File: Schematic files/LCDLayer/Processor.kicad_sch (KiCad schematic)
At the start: 16 parts, among them SW1 SW_SPDT, U5 STM32F103C8Tx, Y1 16MHz

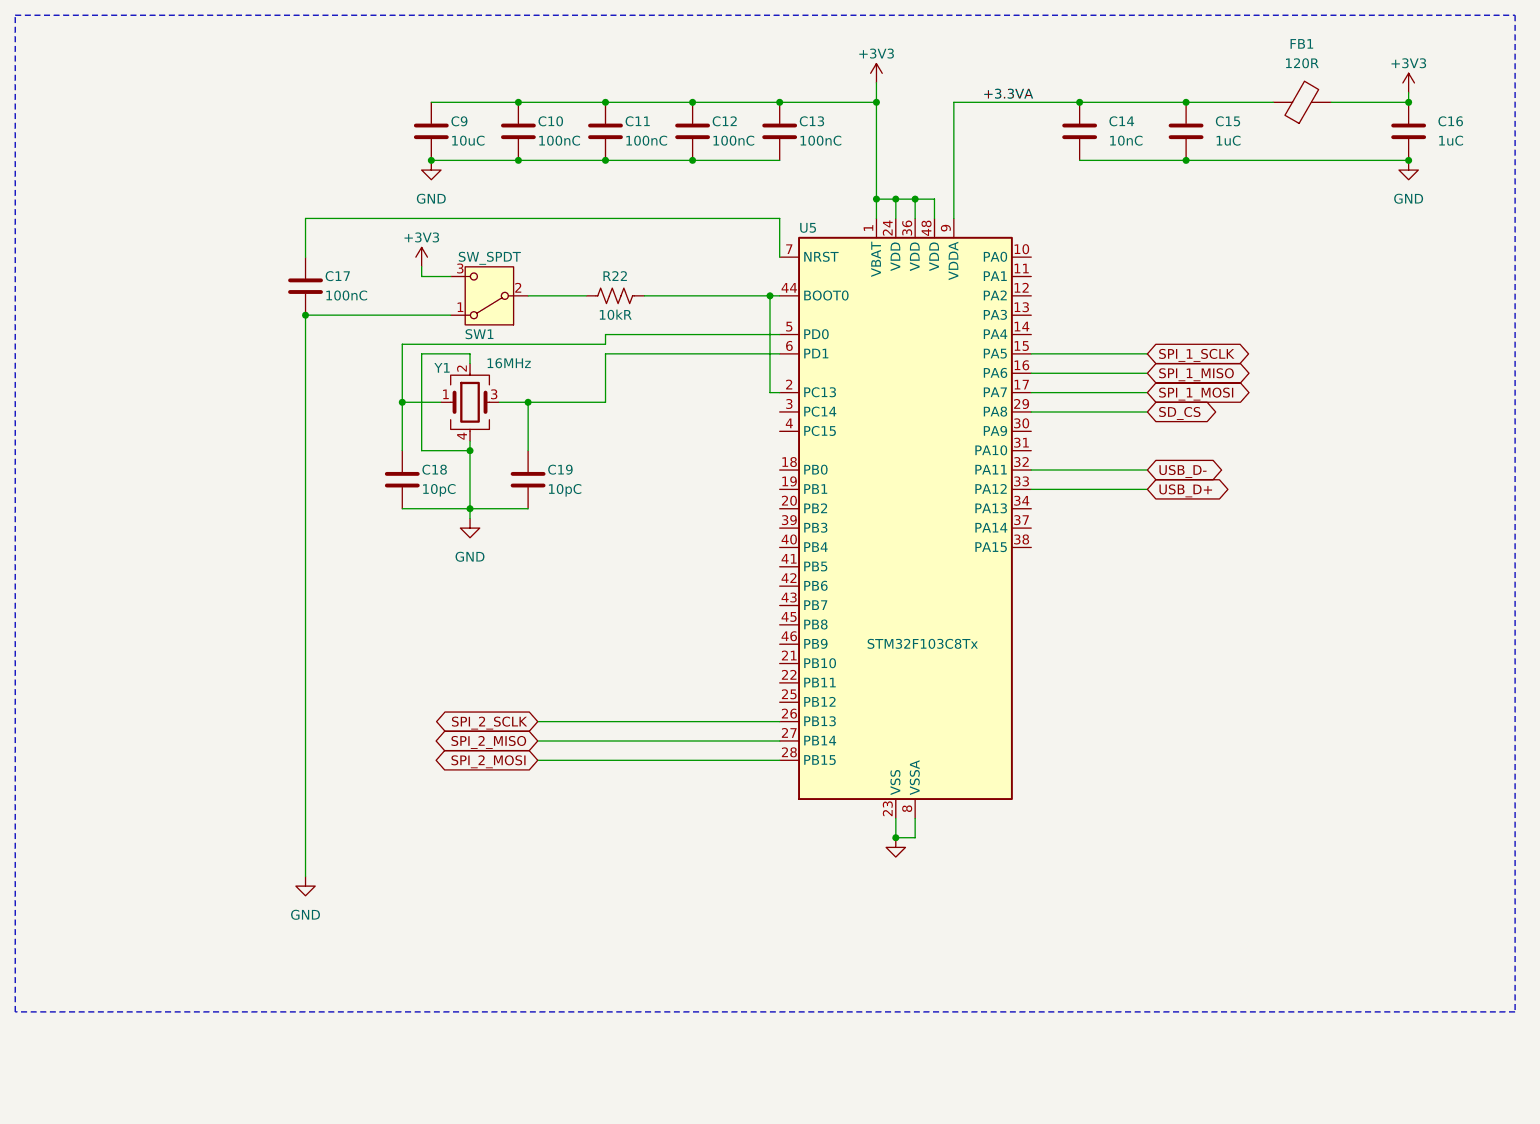
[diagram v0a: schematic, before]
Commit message: Finished Schematic
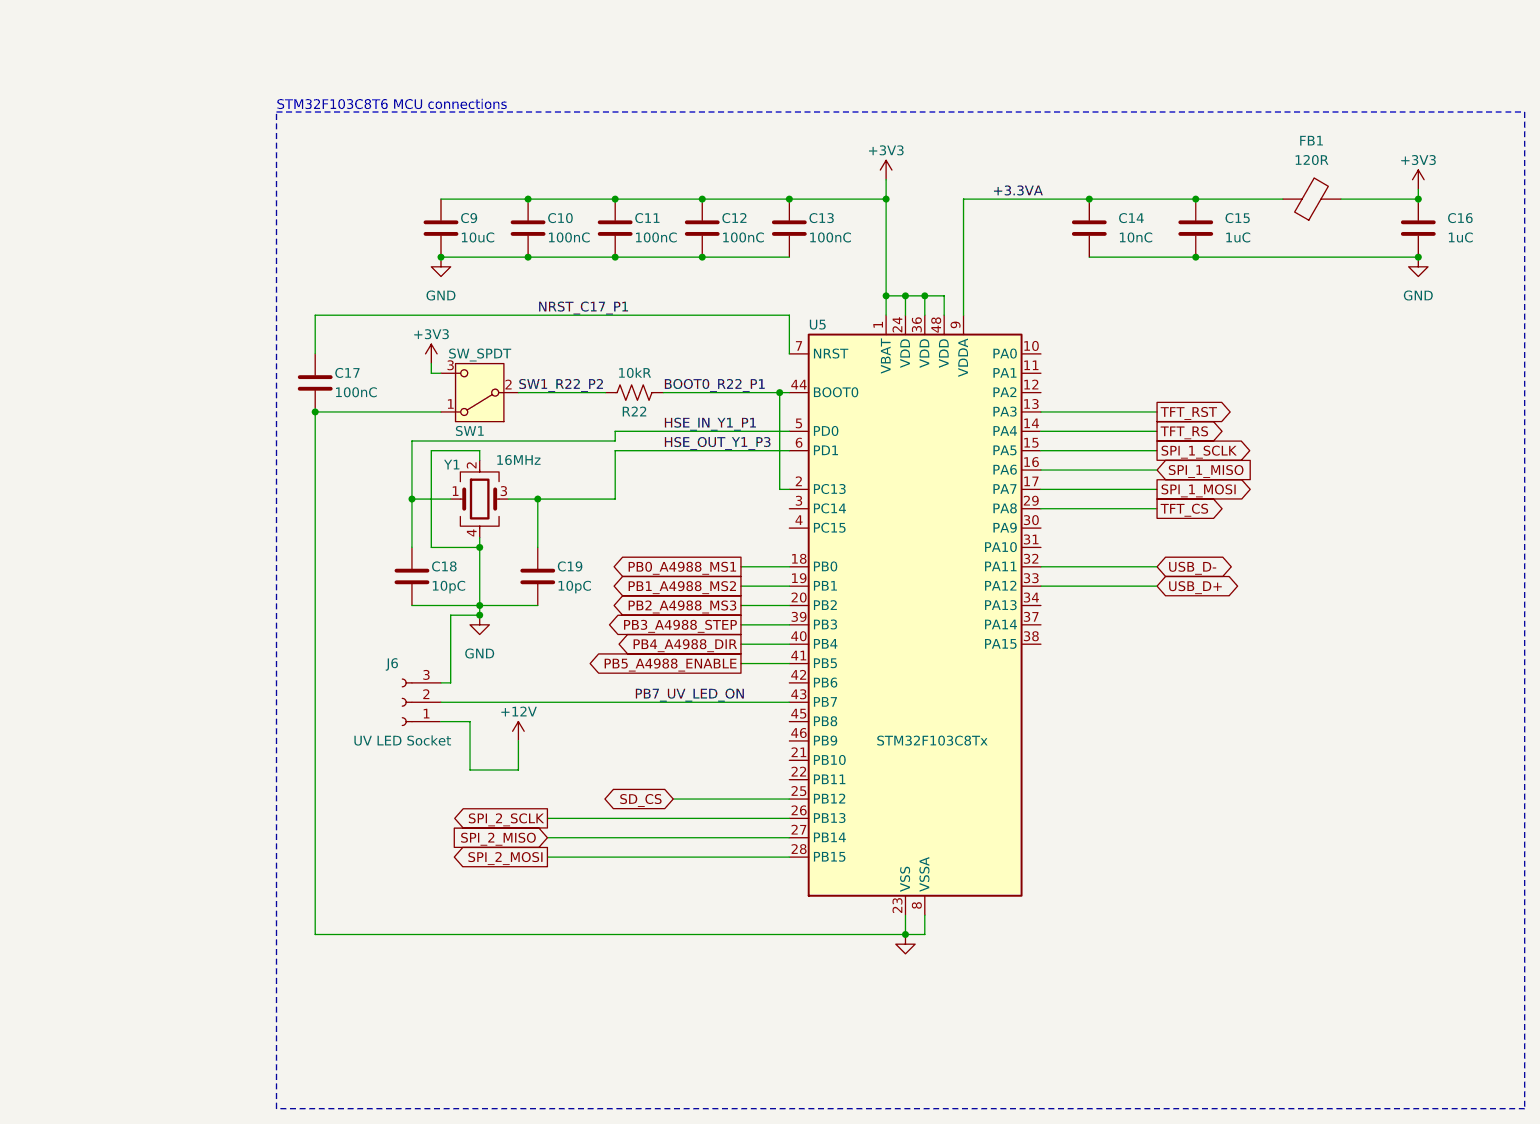
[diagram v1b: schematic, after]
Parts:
- added J6: UV LED Socket, symbol Connector:Conn_01x03_Socket
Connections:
- net GND: now also J6.3 (Pin_3)
- net SD_CS: now also U5.25 (PB12); no longer U5.29 (PA8)
- net BOOT0_R22_P1: now reaches R22.1
- net BOOT0_R22_P1: now also U5.2 (PC13), U5.44 (BOOT0); no longer SW1.2 (B)
- net HSE_IN_Y1_P1: now reaches C18.1, U5.5 (PD0), Y1.1
- net TFT_RST: now reaches U5.13 (PA3)
- net TFT_RS: now reaches U5.14 (PA4)
- net PB0_A4988_MS1: now reaches U5.18 (PB0)
- net PB1_A4988_MS2: now reaches U5.19 (PB1)
- net PB2_A4988_MS3: now reaches U5.20 (PB2)
- net PB3_A4988_STEP: now reaches U5.39 (PB3)
- net PB4_A4988_DIR: now reaches U5.40 (PB4)
- net PB5_A4988_ENABLE: now reaches U5.41 (PB5)
- net PB7_UV_LED_ON: now reaches U5.43 (PB7)
- net PB7_UV_LED_ON: now also J6.2 (Pin_2)
- net HSE_OUT_Y1_P3: now reaches C19.1, U5.6 (PD1), Y1.3
- net NRST_C17_P1: now reaches C17.1, U5.7 (NRST)
- new net +12V: J6.1 (Pin_1)
- new net SW1_R22_P2: R22.2, SW1.2 (B)
- new net TFT_CS: U5.29 (PA8)
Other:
- note added: "STM32F103C8T6 MCU connections"
- company: (none) -> Sidharth Sreeram
- title: (none) -> STM32F103C8T6_MCU
- moved on the sheet: C10, C11, C12, C13, C14, C15, C16, C17, C18, C19, C9, FB1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
